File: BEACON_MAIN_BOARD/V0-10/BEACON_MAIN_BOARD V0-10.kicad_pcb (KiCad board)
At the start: 2 copper layers, 70.4 x 70.4 mm, 114 parts, among them J1001 RJ12, J1002 RJ12, J1003 RJ45, K1001 CONN_3, K1002 CONN_3, K1005 CONN_3, K1006 CONN_3, K1009 USBAB, K1010 COLONETTE, K1011 COLONETTE, K1012 COLONETTE, K1013 COLONETTE, P1001 CONN_5, P1002 CONN_4, P1003 CONN_4, P1004 CONN_4, P1005 CONN_4, Q2001 BSH202, Q2002 2N7002, Q3001 2N7002, Q3002 2N7002, Q3003 2N7002, Q3004 2N7002, Q3005 2N7002, Q3006 2N7002, Q3007 2N7002, Q3008 2N7002, Q3009 2N7002, Q3010 2N7002, SW2001 SW_PUSH_SMALL, SW2002 SWITCH_INV, U2001 PIC24FJ256GB206, U3001 PIC32MX795F512H, X3001 8Mhz

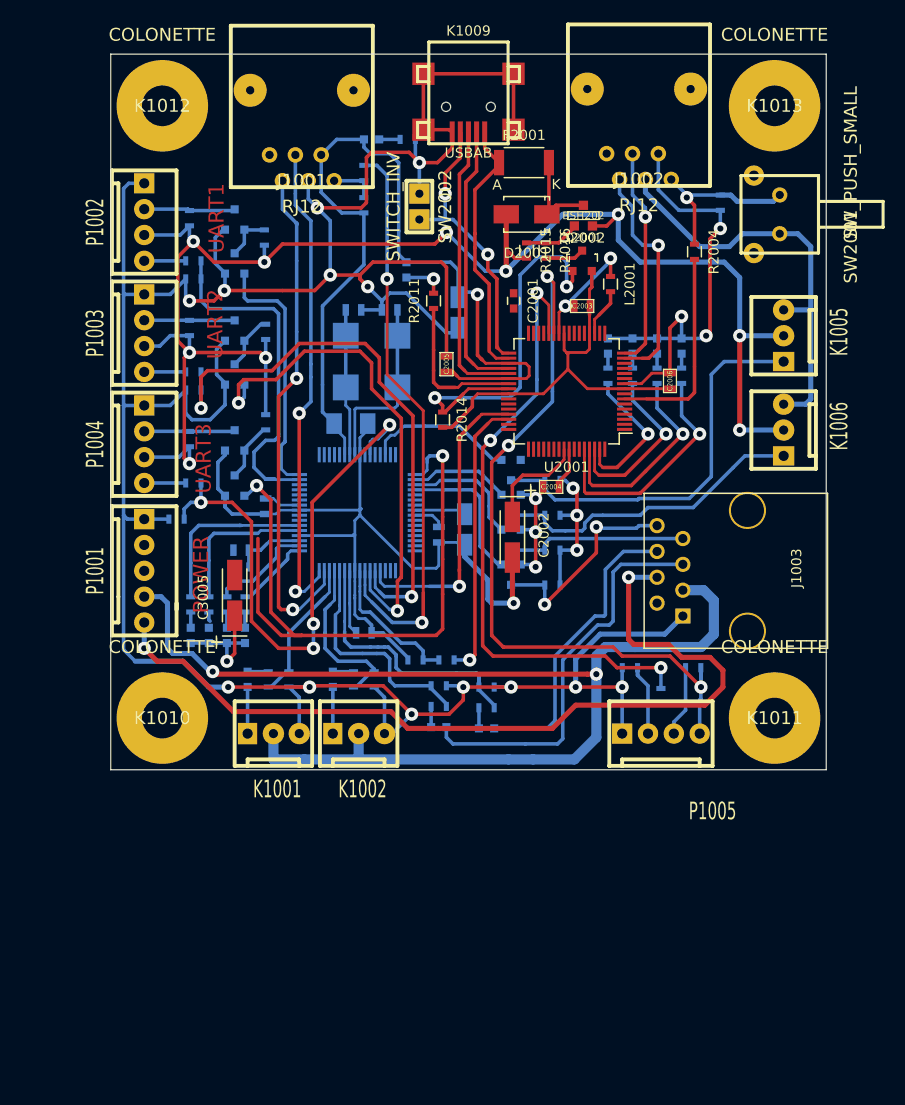
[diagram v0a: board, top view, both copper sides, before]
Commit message: ELECTRONICAL_MAIN_BOARD_32 V1-40
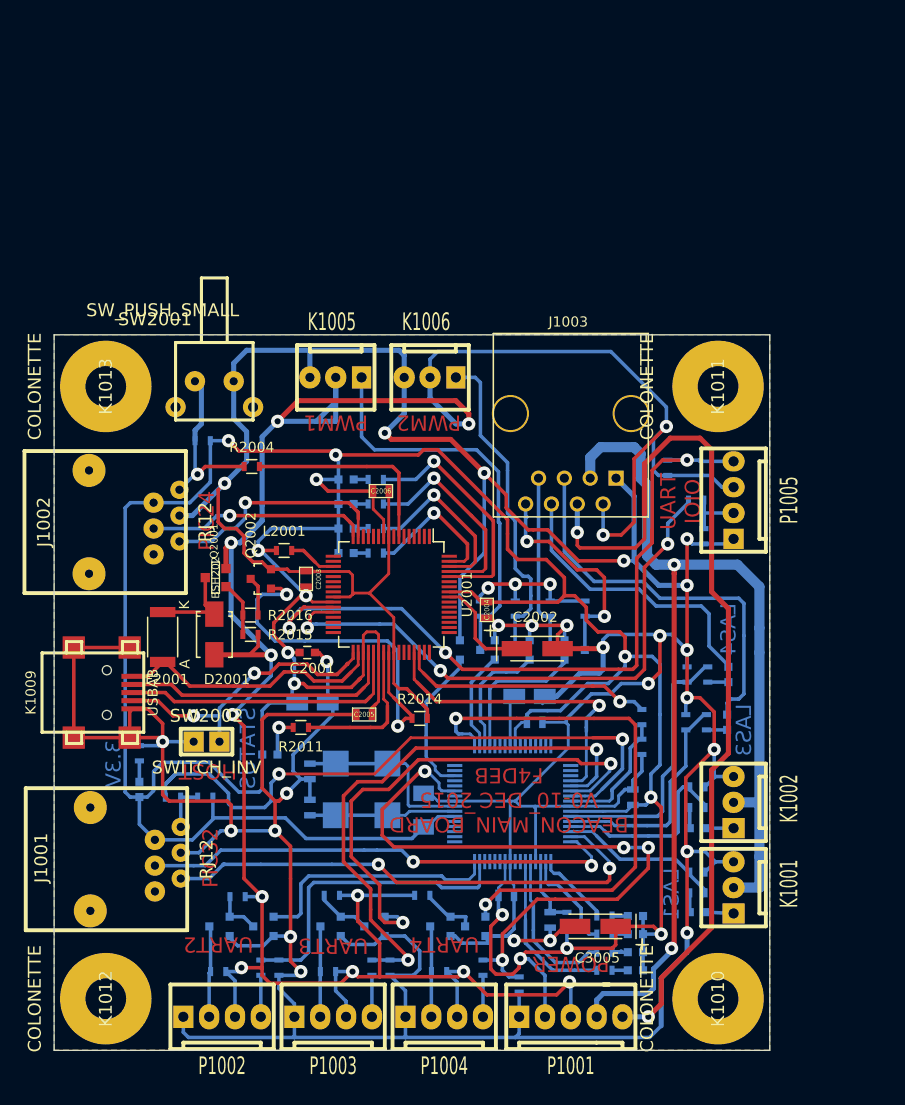
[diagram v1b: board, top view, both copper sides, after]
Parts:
- moved K1012 88.0 mm to (76.2, 151.3), turned to 90 degrees
- moved P1002 75.2 mm to (91.5, 153.1), turned to 180 degrees
- moved R3001 74.1 mm to (87.3, 148.6), turned to 0 degrees
- moved K1013 71.3 mm to (76.2, 91.1), turned to 90 degrees
- moved R3009 69.8 mm to (91.5, 148.2), turned to 270 degrees
- moved K1009 69.6 mm to (75.0, 121.2), turned to 270 degrees
- moved Q3001 69.5 mm to (87.4, 144.2), turned to 270 degrees
- moved R3012 68.2 mm to (93.2, 148.2), turned to 270 degrees
- moved D1009 67.9 mm to (79.5, 130.7), turned to 90 degrees
- moved J1001 67.8 mm to (83.6, 137.6), turned to 270 degrees
- moved P1003 67.2 mm to (102.4, 153.1), turned to 180 degrees
- moved R1001 65.9 mm to (79.5, 127.2), turned to 90 degrees
- moved Q3004 65.2 mm to (91.7, 144.2), turned to 270 degrees
- moved R3004 64.9 mm to (89.2, 141.3), turned to 180 degrees
- moved R3002 64.7 mm to (98.1, 148.6), turned to 0 degrees
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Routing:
- net +3V3: track 176.4 -> 363.9 mm, vias 7 -> 13
- net GND: track 488.7 -> 596.8 mm, vias 17 -> 26
- net +5VD: track 176.4 -> 258.2 mm, vias 10 -> 13
- net Net-(R3011-Pad1): track 78.5 -> 65.4 mm
- net Net-(Q3006-Pad1): track 66.4 -> 53.5 mm
- net Net-(R3015-Pad1): track 57.3 -> 64.4 mm
- net /IOIO/TX4: track 61.8 -> 58.0 mm
- net Net-(R3009-Pad1): track 34.6 -> 31.1 mm
- net +BATT: track 85.5 -> 88.9 mm
- net /IOIO/TX1: track 27.7 -> 25.2 mm
- net Net-(R3026-Pad2): track 16.7 -> 19.1 mm
- net /IOIO/RX424: track 75.0 -> 77.0 mm
- net Net-(R3010-Pad1): track 56.6 -> 54.8 mm
- net Net-(R3024-Pad2): track 14.2 -> 16.0 mm
- net /PIC32MX795F512H/LASER2: track 4.58 -> 2.81 mm
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- added copper zone on B.Cu, net GND
- added copper zone on F.Cu, net GND
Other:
- board text added: "3.3V"
- board text added: "BEACON_MAIN_BOARD V0-10 DEC 2015 F4DEB"
- board text added: "HOST"
- board text added: "LAS1"
- board text added: "LAS3"
- board text added: "LAS4"
- board text added: "PIC24"
- board text added: "PIC32"
- board text added: "PWM1"
- board text added: "PWM2"
- board text added: "STATUS"
- board text added: "UART IOIO"
- board text added: "UART4"
- board text removed: "UART1"
